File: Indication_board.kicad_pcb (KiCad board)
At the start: 2 copper layers, 40 x 110 mm, 17 parts, among them J3 Conn_01x04, J8 Indication, U5 6E1P, U6 6E1P

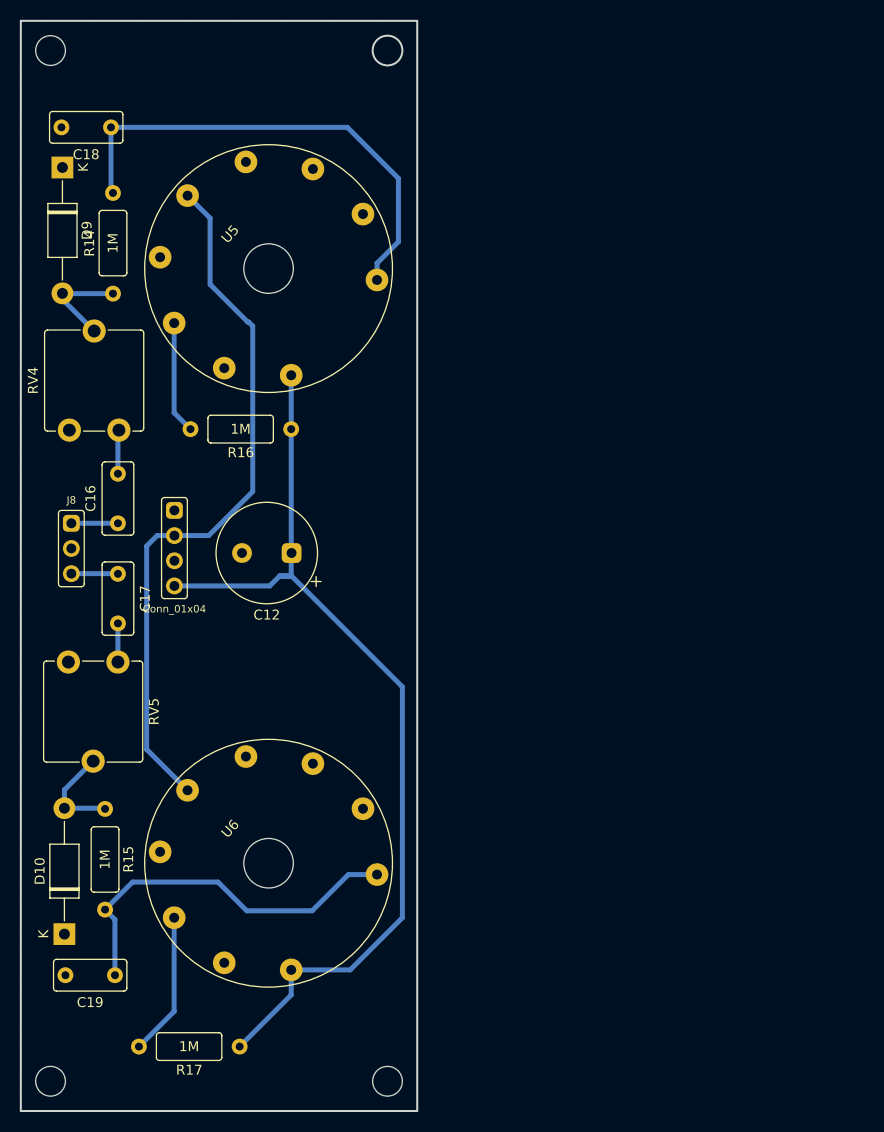
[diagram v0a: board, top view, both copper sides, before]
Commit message: Indication board PCB
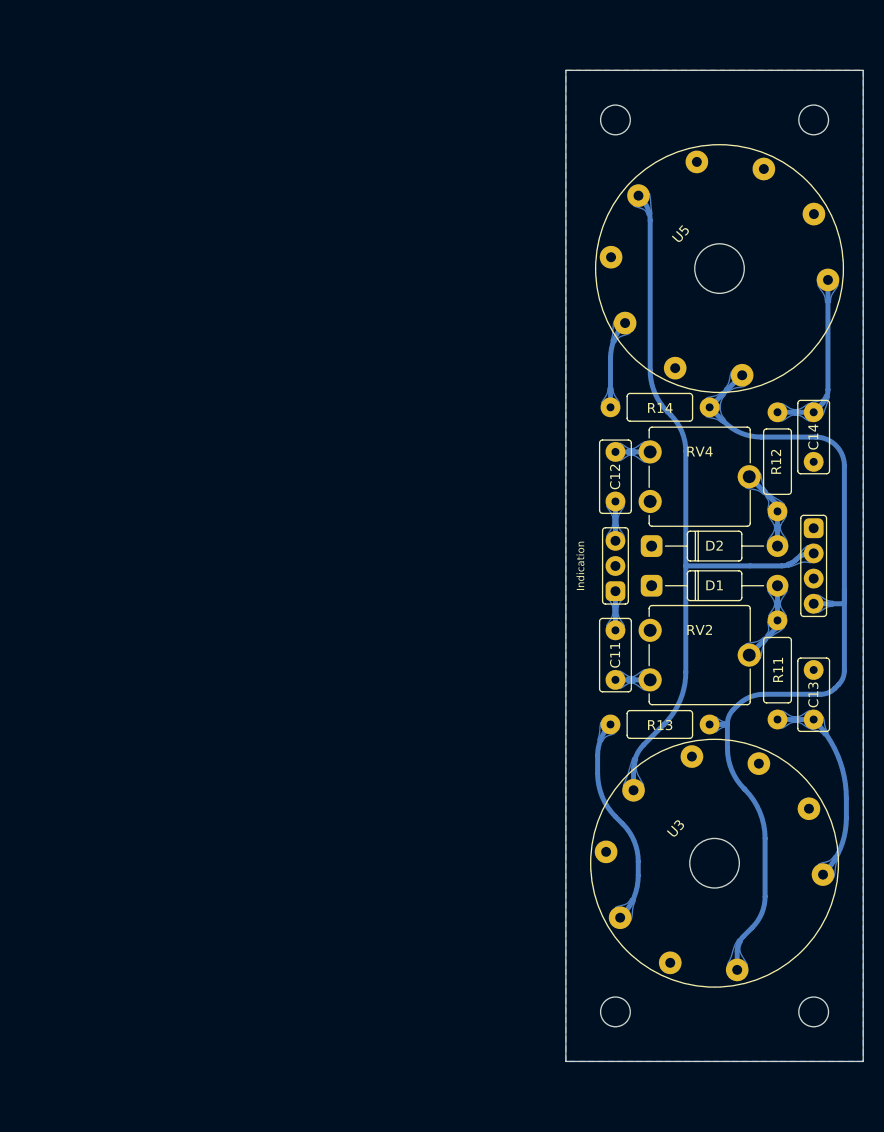
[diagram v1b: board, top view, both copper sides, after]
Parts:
- removed C16, C17, C18, C19: 6800pF, spdf1626_lib:C_THT_K73-17_P5.00mm
- removed D10, D9: 1n4007, Diode_THT:D_DO-41_SOD81_P12.70mm_Horizontal
- removed J3: Conn_01x04, spdf1626_lib:PinHeader_1x04_P2.54mm
- removed J8: Indication, spdf1626_lib:PinHeader_1x03_P2.54mm
- removed R15, R16, R17: 1M, spdf1626_lib:R_THT_025W
- removed RV5: 470k, spdf1626_lib:Potentiometer_THT_CA9V
- removed U6: 6E1P, spdf1626_lib:9-pin_tube_socket
- added C11: 6800pF, spdf1626_lib:C_THT_K73-17_P5.00mm, F.Cu at (135.0, 76.5)
- added C13: 6800pF, spdf1626_lib:C_THT_K73-17_P5.00mm, F.Cu at (155.0, 85.5)
- added C14: 6800pF, spdf1626_lib:C_THT_K73-17_P5.00mm, F.Cu at (155.0, 54.5)
- added D1: 1n4007, spdf1626_lib:D_DO-41, F.Cu at (138.7, 72.0)
- added D2: 1n4007, spdf1626_lib:D_DO-41, F.Cu at (138.7, 68.0)
- added J4: Indication, spdf1626_lib:PinHeader_1x03_P2.54mm, F.Cu at (135.0, 72.5)
- added J5: Conn_01x04, spdf1626_lib:PinHeader_1x04_P2.54mm, F.Cu at (155.0, 66.2)
- added R11: 1M, spdf1626_lib:R_THT_025W, F.Cu at (151.3, 80.5)
- added R12: 1M, spdf1626_lib:R_THT_025W, F.Cu at (151.3, 59.5)
- added R13: 1M, spdf1626_lib:R_THT_025W, F.Cu at (139.5, 86.0)
- added RV2: 470k, spdf1626_lib:Potentiometer_THT_CA9V, F.Cu at (138.5, 81.5)
- added U3: 6E1P, spdf1626_lib:9-pin_tube_socket, F.Cu at (145.0, 100.0)
- C12: value 10uF -> 6800pF; footprint spdf1626_lib:C_THT_D10.0mm_P5.00mm -> spdf1626_lib:C_THT_K73-17_P5.00mm
- moved R14 56.4 mm to (139.5, 54.0), turned to 180 degrees
- moved RV4 54.1 mm to (138.5, 63.5), turned to 0 degrees
- moved U5 45.5 mm to (145.5, 40.0)
- moved C12 33.1 mm to (135.0, 63.5), turned to 90 degrees
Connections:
- C12 pad 1: 240V -> Net-(C12-Pad1)
- C12 pad 2: GND -> Net-(C12-Pad2)
- R14 pad 1: Net-(D9-Pad2) -> 240V
- R14 pad 2: Net-(C18-Pad1) -> Net-(R14-Pad2)
- RV4 pad 1: Net-(C16-Pad2) -> GND
- RV4 pad 2: Net-(D9-Pad2) -> Net-(D2-Pad2)
- RV4 pad 3: GND -> Net-(C12-Pad2)
- U5 pad 1: Net-(C18-Pad1) -> Net-(C14-Pad1)
- U5 pad 7: Net-(R16-Pad2) -> Net-(R14-Pad2)
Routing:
- net Net-(C18-Pad1): track 49.0 -> 0.00 mm
- net Net-(C19-Pad1): track 38.3 -> 0.00 mm
- net Net-(R13-Pad2): track 0.00 -> 21.4 mm
- net Net-(C13-Pad1): track 0.00 -> 20.7 mm
- net Net-(C14-Pad1): track 0.00 -> 17.5 mm
- net Net-(R17-Pad2): track 14.5 -> 0.00 mm
- net Net-(R16-Pad2): track 11.5 -> 0.00 mm
- net Net-(D9-Pad2): track 10.2 -> 0.00 mm
- net Net-(D10-Pad2): track 10.1 -> 0.00 mm
- net Net-(R14-Pad2): track 0.00 -> 8.87 mm
- net Net-(D1-Pad2): track 0.00 -> 8.18 mm
- net Net-(D2-Pad2): track 0.00 -> 8.18 mm
- net 240V: track 96.1 -> 88.8 mm
- net Net-(C17-Pad1): track 4.71 -> 0.00 mm
- net Net-(C16-Pad1): track 4.70 -> 0.00 mm
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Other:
- board size 40 x 110 mm -> 30 x 100 mm
